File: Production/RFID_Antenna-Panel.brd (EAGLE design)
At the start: 97.3 x 63.2 mm, 75 parts, among them J1 U.FL, J2 U.FL, J3 U.FL

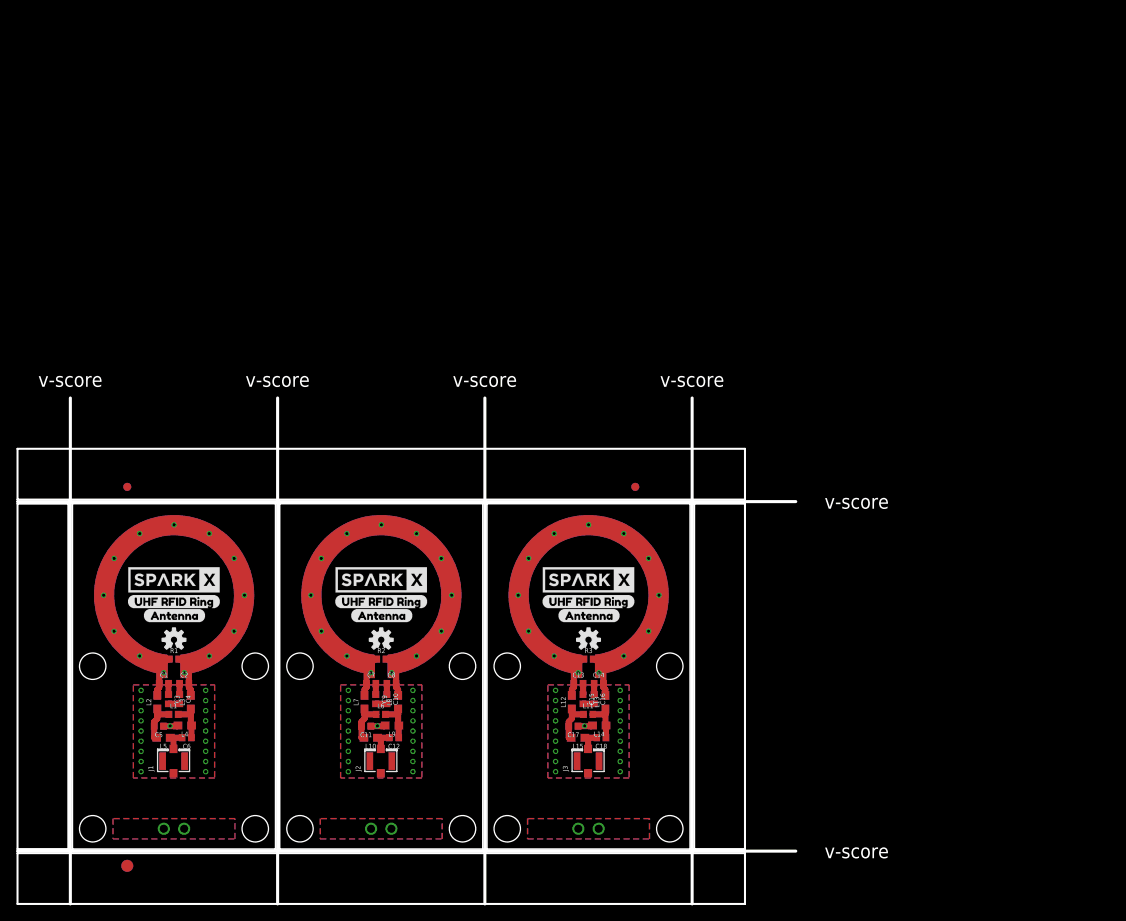
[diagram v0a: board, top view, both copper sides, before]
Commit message: Caopy Murata Design w/ Transparency for x02
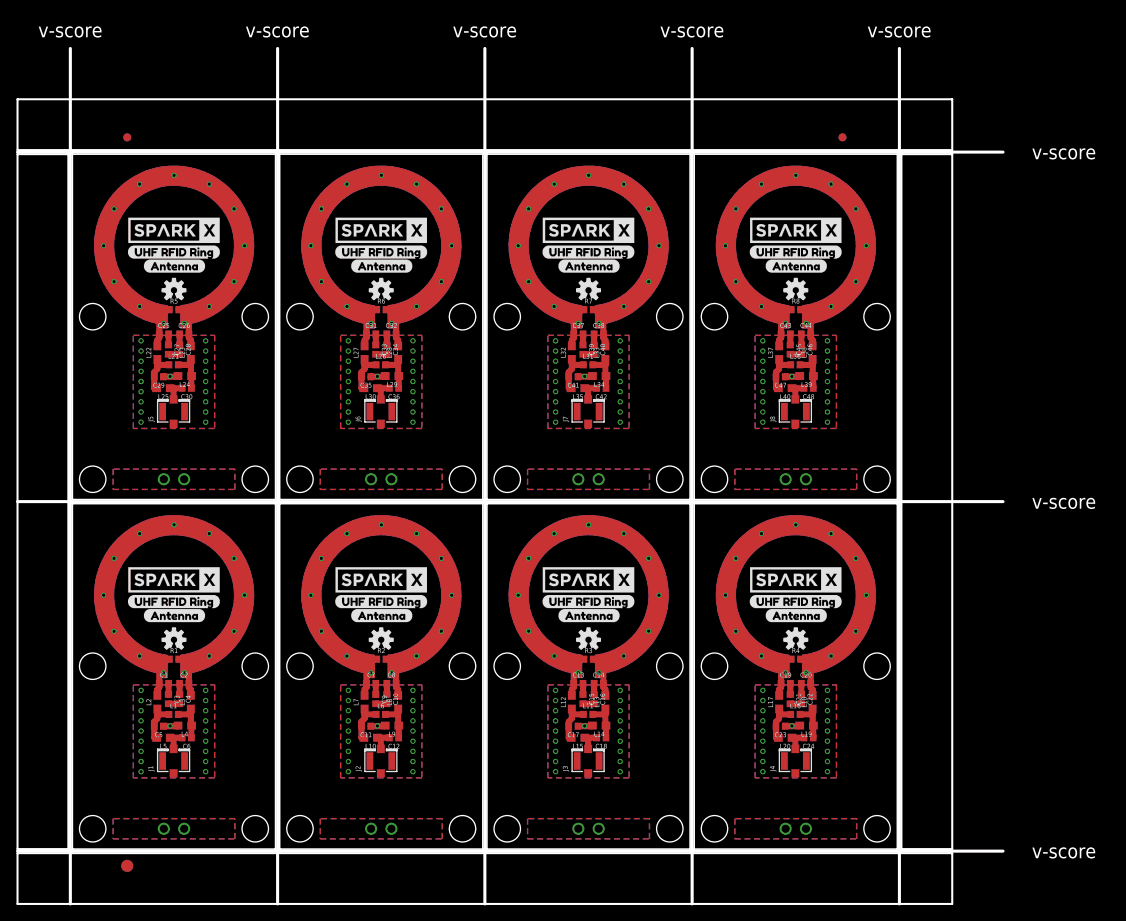
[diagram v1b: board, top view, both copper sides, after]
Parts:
- added C19, C20, C25, C26, C31, C32, C37, C38, C43, C44: 9.3 pF, special_parts:0402
- added C21, C22, C27, C28, C33, C34, C39, C40, C45, C46: 9.0 pF, special_parts:0402
- added C23, C24, C29, C30, C35, C36, C41, C42, C47, C48: 5.66 pF, special_parts:0402
- added J4, J5, J6, J7, J8: U.FL, SparkFun-Connectors:U.FL
- added L16, L21, L26, L31, L36: 0.26 uH, special_parts:0402
- added L17, L18, L22, L23, L27, L28, L32, L33, L37, L38: 0.26 uH, special_parts:0603
- added L19, L20, L24, L25, L29, L30, L34, L35, L39, L40: 0.24 uH, special_parts:0603
- added R4, R5, R6, R7, R8: 4.28k, special_parts:0402
- added U$31, U$41, U$51, U$61, U$71: ANTENNA, special_parts:ANT
- added U$32, U$33, U$42, U$43, U$52, U$53, U$62, U$63, U$72, U$73: (no value), SparkX:SPARKX-LARGE
- added U$34, U$35, U$44, U$45, U$54, U$55, U$64, U$65, U$74, U$75: (no value), buzzard_labels:UHF_RFID_RING0
- added U$36, U$37, U$46, U$47, U$56, U$57, U$66, U$67, U$76, U$77: (no value), buzzard_labels:ANTENNA1
- added U$38, U$39, U$48, U$49, U$58, U$59, U$68, U$69, U$78, U$79: (no value), SparkFun-Aesthetics:OSHW-LOGO-S
- added U$40, U$50, U$60, U$70, U$80: (no value), SparkX:QWIIC_BOARD_MOUNT_HOLES
- moved E$3 50.8 mm to (96.3, 89.0)
- moved E$4 50.8 mm to (96.3, 89.0)
- moved E$1 43.7 mm to (6.86, 89.0)
- moved E$2 43.7 mm to (6.86, 89.0)
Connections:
- new net A10: C26.2, L23.2, R5.2, U$41.P$2, U$41.P$4
- new net A11: C31.1, L27.2, R6.1, U$51.P$1, U$51.P$3
- new net A12: C32.2, L28.2, R6.2, U$51.P$2, U$51.P$4
- new net A13: C37.1, L32.2, R7.1, U$61.P$1, U$61.P$3
- new net A14: C38.2, L33.2, R7.2, U$61.P$2, U$61.P$4
- new net A15: C43.1, L37.2, R8.1, U$71.P$1, U$71.P$3
- new net A16: C44.2, L38.2, R8.2, U$71.P$2, U$71.P$4
- new net A7: C19.1, L17.2, R4.1, U$31.P$1, U$31.P$3
- new net A8: C20.2, L18.2, R4.2, U$31.P$2, U$31.P$4
- new net A9: C25.1, L22.2, R5.1, U$41.P$1, U$41.P$3
- new net C1C4: C19.2, C21.1
- new net C1C5: C25.2, C27.1
- new net C1C6: C31.2, C33.1
- new net C1C7: C37.2, C39.1
- new net C1C8: C43.2, C45.1
- new net C2C3: C20.1, C22.1
- new net C2C5: C26.1, C28.1
- new net C2C6: C32.1, C34.1
- new net C2C7: C38.1, C40.1
- new net C2C8: C44.1, C46.1
- new net C3C3: C21.2, C22.2
- new net C3C5: C27.2, C28.2
- new net C3C6: C33.2, C34.2
- new net C3C7: C39.2, C40.2
- new net C3C8: C45.2, C46.2
- new net GND10: C35.1, J6.1, J6.2, L29.2
- new net GND12: C41.1, J7.1, J7.2, L34.2
- new net GND14: C47.1, J8.1, J8.2, L39.2
- new net GND6: C23.1, J4.1, J4.2, L19.2
- new net GND8: C29.1, J5.1, J5.2, L24.2
- new net L5C3: C24.2, J4.FEED, L20.1
- new net L5C4: C30.2, J5.FEED, L25.1
- new net L5C5: C36.2, J6.FEED, L30.1
- new net L5C7: C42.2, J7.FEED, L35.1
- new net L5C8: C48.2, J8.FEED, L40.1
- new net N$106: C48.1, L36.2, L38.1, L39.1
- new net N$107: C47.2, L36.1, L37.1, L40.2
- new net N$46: C24.1, L16.2, L18.1, L19.1
- new net N$47: C23.2, L16.1, L17.1, L20.2
- new net N$61: C30.1, L21.2, L23.1, L24.1
- new net N$62: C29.2, L21.1, L22.1, L25.2
- new net N$76: C36.1, L26.2, L28.1, L29.1
- new net N$77: C35.2, L26.1, L27.1, L30.2
- new net N$91: C42.1, L31.2, L33.1, L34.1
- new net N$92: C41.2, L31.1, L32.1, L35.2
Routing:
- net N$46: track 0.00 -> 5.93 mm
- net N$106: track 0.00 -> 5.93 mm
- net N$76: track 0.00 -> 5.93 mm
- net N$91: track 0.00 -> 5.93 mm
- net N$61: track 0.00 -> 5.93 mm
- net A16: track 0.00 -> 5.61 mm
- net A8: track 0.00 -> 5.61 mm
- net A12: track 0.00 -> 5.61 mm
- net A10: track 0.00 -> 5.61 mm
- net A14: track 0.00 -> 5.61 mm
- net A13: track 0.00 -> 5.55 mm
- net A11: track 0.00 -> 5.55 mm
- net A9: track 0.00 -> 5.55 mm
- net A7: track 0.00 -> 5.55 mm
- net A15: track 0.00 -> 5.55 mm
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- added copper zone on layer 1, net GND10
- added copper zone on layer 16, net GND10
- added copper zone on layer 1, net GND11
- added copper zone on layer 16, net GND11
- added copper zone on layer 1, net GND12
- added copper zone on layer 16, net GND12
- added copper zone on layer 1, net GND13
- added copper zone on layer 16, net GND13
- added copper zone on layer 1, net GND14
- added copper zone on layer 16, net GND14
- added copper zone on layer 1, net GND15
- added copper zone on layer 16, net GND15
- added copper zone on layer 1, net GND6
- added copper zone on layer 16, net GND6
- added copper zone on layer 1, net GND7
- added copper zone on layer 16, net GND7
- added copper zone on layer 1, net GND8
- added copper zone on layer 16, net GND8
- added copper zone on layer 1, net GND9
- added copper zone on layer 16, net GND9
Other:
- board size 97.3 x 63.2 mm -> 123.2 x 106.9 mm

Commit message: Add production for x02
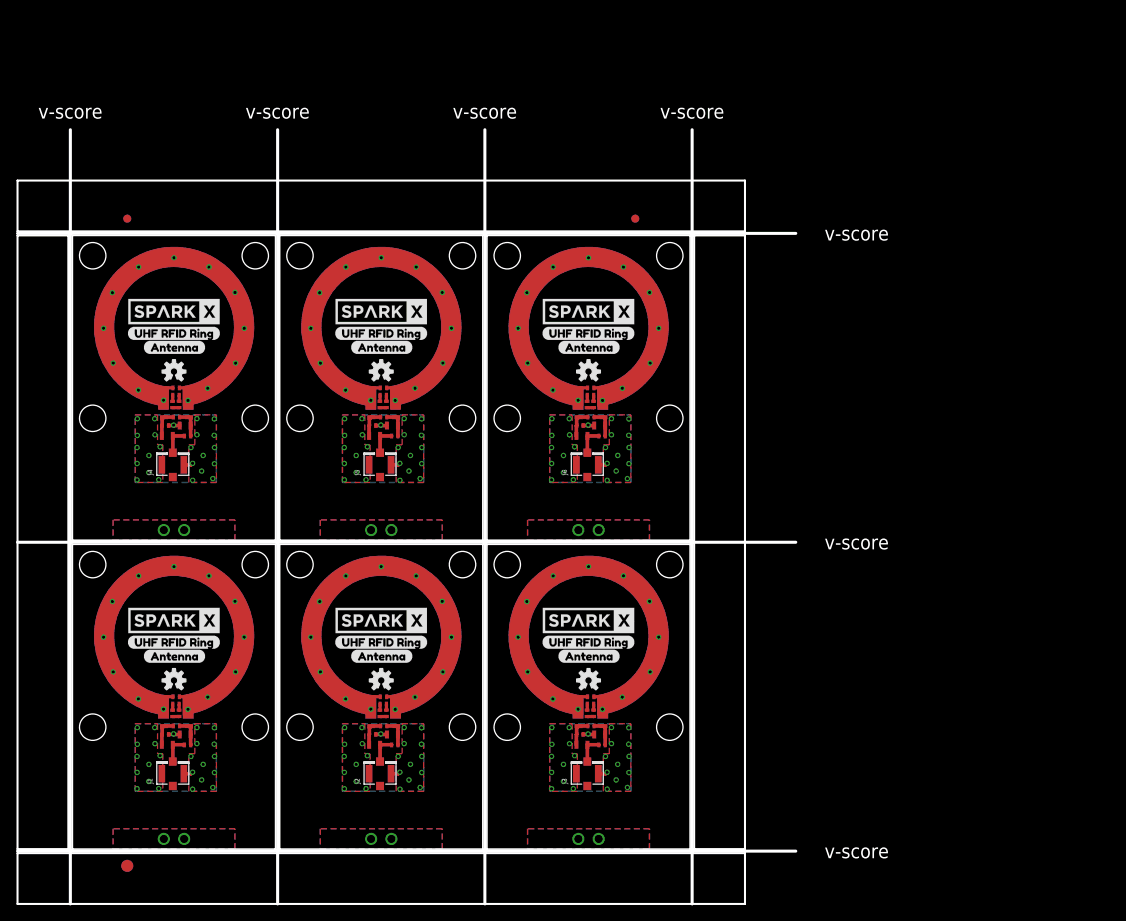
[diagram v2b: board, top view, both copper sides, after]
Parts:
- removed C37, C38, C43, C44: 9.3 pF, special_parts:0402
- removed C39, C40, C45, C46: 9.0 pF, special_parts:0402
- removed C41, C42, C47, C48: 5.66 pF, special_parts:0402
- removed J7, J8: U.FL, SparkFun-Connectors:U.FL
- removed L31, L36: 0.26 uH, special_parts:0402
- removed L32, L33, L37, L38: 0.26 uH, special_parts:0603
- removed L34, L35, L39, L40: 0.24 uH, special_parts:0603
- removed R7, R8: 4.28k, special_parts:0402
- removed U$61, U$71: ANTENNA, special_parts:ANT
- removed U$62, U$63, U$72, U$73: (no value), SparkX:SPARKX-LARGE
- removed U$64, U$65, U$74, U$75: (no value), buzzard_labels:UHF_RFID_RING0
- removed U$66, U$67, U$76, U$77: (no value), buzzard_labels:ANTENNA1
- removed U$68, U$69, U$78, U$79: (no value), SparkFun-Aesthetics:OSHW-LOGO-S
- removed U$70, U$80: (no value), SparkX:QWIIC_BOARD_MOUNT_HOLES
- C1, C10, C11, C12, C13, C14, C15, C16, C17, C18, C19, C2, C20, C21, C22, C23, C24, C25, C26, C27, C28, C29, C3, C30, C31, C32, C33, C34, C35, C36, C4, C5, C6, C7, C8, C9, L1, L11, L16, L21, L26, L6, R1, R2, R3, R4, R5, R6: device special_parts:0402 -> special_parts:0402_MURATA
- L10, L12, L13, L14, L15, L17, L18, L19, L2, L20, L22, L23, L24, L25, L27, L28, L29, L3, L30, L4, L5, L7, L8, L9: device special_parts:0603 -> special_parts:0603_MURATA
- moved U$40 93.1 mm to (12.7, 64.0)
- moved C24 86.3 mm to (14.4, 51.6)
- moved L19 86.3 mm to (14.1, 52.9)
- moved J4 86.2 mm to (12.5, 48.0)
- moved C22 86.1 mm to (13.3, 55.6)
- moved L18 86.0 mm to (14.6, 54.7)
- moved L20 86.0 mm to (11.9, 51.6)
- moved C20 85.9 mm to (13.7, 56.7)
- moved L16 85.8 mm to (13.0, 54.0)
- moved C23 85.6 mm to (11.6, 52.9)
- moved C21 85.6 mm to (12.5, 55.6)
- moved C19 85.0 mm to (12.1, 56.7)
- moved L17 85.0 mm to (11.4, 54.7)
- moved U$32 84.6 mm to (12.7, 67.2)
- moved U$33 84.6 mm to (12.7, 67.2)
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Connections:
- removed net A13: C37.1, L32.2, R7.1, U$61.P$1, U$61.P$3
- removed net A14: C38.2, L33.2, R7.2, U$61.P$2, U$61.P$4
- removed net A15: C43.1, L37.2, R8.1, U$71.P$1, U$71.P$3
- removed net A16: C44.2, L38.2, R8.2, U$71.P$2, U$71.P$4
- removed net C1C7: C37.2, C39.1
- removed net C1C8: C43.2, C45.1
- removed net C2C7: C38.1, C40.1
- removed net C2C8: C44.1, C46.1
- removed net C3C7: C39.2, C40.2
- removed net C3C8: C45.2, C46.2
- removed net GND12: C41.1, J7.1, J7.2, L34.2
- removed net GND14: C47.1, J8.1, J8.2, L39.2
- removed net L5C7: C42.2, J7.FEED, L35.1
- removed net L5C8: C48.2, J8.FEED, L40.1
- removed net N$106: C48.1, L36.2, L38.1, L39.1
- removed net N$107: C47.2, L36.1, L37.1, L40.2
- removed net N$16: C12.1, L6.2, L8.1, L9.1
- removed net N$17: C11.2, L10.2, L6.1, L7.1
- removed net N$31: C18.1, L11.2, L13.1, L14.1
- removed net N$32: C17.2, L11.1, L12.1, L15.2
- removed net N$91: C42.1, L31.2, L33.1, L34.1
- removed net N$92: C41.2, L31.1, L32.1, L35.2
- new net N$1: C12.P$1, L6.P$2, L8.P$1, L9.P$1
- new net N$18: C18.P$1, L11.P$2, L13.P$1, L14.P$1
- new net N$19: C17.P$2, L11.P$1, L12.P$1, L15.P$2
- new net N$2: C11.P$2, L10.P$2, L6.P$1, L7.P$1
- net A1: now also C1.P$1, L2.P$2, R1.P$1; no longer C1.1, L2.2, R1.1
- net A10: now also C26.P$2, L23.P$2, R5.P$2; no longer C26.2, L23.2, R5.2
- net A11: now also C31.P$1, L27.P$2, R6.P$1; no longer C31.1, L27.2, R6.1
- net A12: now also C32.P$2, L28.P$2, R6.P$2; no longer C32.2, L28.2, R6.2
- net A2: now also C2.P$2, L3.P$2, R1.P$2; no longer C2.2, L3.2, R1.2
- net A3: now also C7.P$1, L7.P$2, R2.P$1; no longer C7.1, L7.2, R2.1
- net A4: now also C8.P$2, L8.P$2, R2.P$2; no longer C8.2, L8.2, R2.2
- net A5: now also C13.P$1, L12.P$2, R3.P$1; no longer C13.1, L12.2, R3.1
- net A6: now also C14.P$2, L13.P$2, R3.P$2; no longer C14.2, L13.2, R3.2
- net A7: now also C19.P$1, L17.P$2, R4.P$1; no longer C19.1, L17.2, R4.1
- net A8: now also C20.P$2, L18.P$2, R4.P$2; no longer C20.2, L18.2, R4.2
- net A9: now also C25.P$1, L22.P$2, R5.P$1; no longer C25.1, L22.2, R5.1
- net C1C1: now also C7.P$2, C9.P$1; no longer C7.2, C9.1
- net C1C2: now also C13.P$2, C15.P$1; no longer C13.2, C15.1
- net C1C3: now also C1.P$2, C3.P$1; no longer C1.2, C3.1
- net C1C4: now also C19.P$2, C21.P$1; no longer C19.2, C21.1
- net C1C5: now also C25.P$2, C27.P$1; no longer C25.2, C27.1
- net C1C6: now also C31.P$2, C33.P$1; no longer C31.2, C33.1
- net C2C1: now also C10.P$1, C8.P$1; no longer C10.1, C8.1
- net C2C2: now also C14.P$1, C16.P$1; no longer C14.1, C16.1
- net C2C3: now also C20.P$1, C22.P$1; no longer C20.1, C22.1
- net C2C4: now also C2.P$1, C4.P$1; no longer C2.1, C4.1
- net C2C5: now also C26.P$1, C28.P$1; no longer C26.1, C28.1
- net C2C6: now also C32.P$1, C34.P$1; no longer C32.1, C34.1
- net C3C1: now also C10.P$2, C9.P$2; no longer C10.2, C9.2
- net C3C2: now also C15.P$2, C16.P$2; no longer C15.2, C16.2
- net C3C3: now also C21.P$2, C22.P$2; no longer C21.2, C22.2
- net C3C4: now also C3.P$2, C4.P$2; no longer C3.2, C4.2
- net C3C5: now also C27.P$2, C28.P$2; no longer C27.2, C28.2
- net C3C6: now also C33.P$2, C34.P$2; no longer C33.2, C34.2
- net GND: now also C5.P$1, L4.P$2; no longer C5.1, L4.2
- net GND10: now also C35.P$1, L29.P$2; no longer C35.1, L29.2
- net GND2: now also C11.P$1, L9.P$2; no longer C11.1, L9.2
- net GND4: now also C17.P$1, L14.P$2; no longer C17.1, L14.2
- net GND6: now also C23.P$1, L19.P$2; no longer C23.1, L19.2
- net GND8: now also C29.P$1, L24.P$2; no longer C29.1, L24.2
- net L5C1: now also C12.P$2, L10.P$1; no longer C12.2, L10.1
- net L5C2: now also C18.P$2, L15.P$1; no longer C18.2, L15.1
- net L5C3: now also C24.P$2, L20.P$1; no longer C24.2, L20.1
- net L5C4: now also C30.P$2, L25.P$1; no longer C30.2, L25.1
- net L5C5: now also C36.P$2, L30.P$1; no longer C36.2, L30.1
- net L5C6: now also C6.P$2, L5.P$1; no longer C6.2, L5.1
- net N$46: now also C24.P$1, L16.P$2, L18.P$1, L19.P$1; no longer C24.1, L16.2, L18.1, L19.1
- net N$47: now also C23.P$2, L16.P$1, L17.P$1, L20.P$2; no longer C23.2, L16.1, L17.1, L20.2
- net N$6: now also C6.P$1, L1.P$2, L3.P$1, L4.P$1; no longer C6.1, L1.2, L3.1, L4.1
- net N$61: now also C30.P$1, L21.P$2, L23.P$1, L24.P$1; no longer C30.1, L21.2, L23.1, L24.1
- net N$62: now also C29.P$2, L21.P$1, L22.P$1, L25.P$2; no longer C29.2, L21.1, L22.1, L25.2
- net N$7: now also C5.P$2, L1.P$1, L2.P$1, L5.P$2; no longer C5.2, L1.1, L2.1, L5.2
- net N$76: now also C36.P$1, L26.P$2, L28.P$1, L29.P$1; no longer C36.1, L26.2, L28.1, L29.1
- net N$77: now also C35.P$2, L26.P$1, L27.P$1, L30.P$2; no longer C35.2, L26.1, L27.1, L30.2
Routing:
- net N$106: track 5.93 -> 0.00 mm
- net N$16: track 5.93 -> 0.00 mm, vias 0 -> 1
- net N$91: track 5.93 -> 0.00 mm
- net N$31: track 5.93 -> 0.00 mm, vias 0 -> 1
- net A16: track 5.61 -> 0.00 mm
- net A14: track 5.61 -> 0.00 mm
- net A13: track 5.55 -> 0.00 mm
- net A15: track 5.55 -> 0.00 mm
- net N$107: track 5.50 -> 0.00 mm
- net N$17: track 5.50 -> 0.00 mm, vias 0 -> 1
- net N$32: track 5.50 -> 0.00 mm, vias 0 -> 1
- net N$92: track 5.50 -> 0.00 mm
- net A5: track 5.55 -> 1.44 mm
- net A11: track 5.55 -> 1.44 mm
- net A3: track 5.55 -> 1.44 mm
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- removed copper zone on layer 1, net GND12
- removed copper zone on layer 16, net GND12
- removed copper zone on layer 1, net GND13
- removed copper zone on layer 16, net GND13
- removed copper zone on layer 1, net GND14
- removed copper zone on layer 16, net GND14
- removed copper zone on layer 1, net GND15
- removed copper zone on layer 16, net GND15
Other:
- board size 123.2 x 106.9 mm -> 97.3 x 96.8 mm
